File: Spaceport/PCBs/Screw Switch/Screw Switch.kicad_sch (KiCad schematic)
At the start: 2 parts

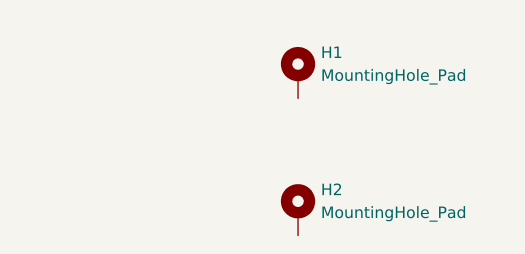
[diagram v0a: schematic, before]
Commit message: Update Screw Switch PCB and schematic files
- Increased pad dimensions in Screw Switch PCB from 3.8mm to 9.0mm for improved soldering and stability.
- Added a new mounting hole symbol in the Screw Switch schematic with properties for reference, value, footprint, datasheet, and description.
- Created an auto-saved file entry for the STM32 flight computer project to ensure recovery of recent changes.
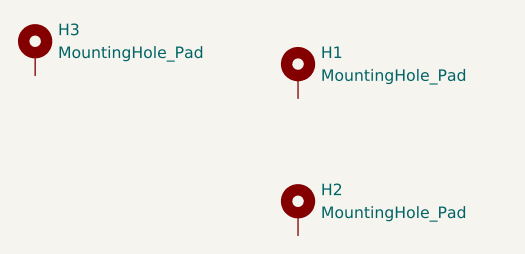
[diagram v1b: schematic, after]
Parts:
- added H3: MountingHole_Pad, MountingHole:MountingHole_3.2mm_M3_Pad_TopBottom, symbol Mechanical:MountingHole_Pad
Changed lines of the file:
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@@
+	(symbol
+		(lib_id "Mechanical:MountingHole_Pad")
+		(at 82.55 68.58 0)
+		(unit 1)
+		(exclude_from_sim yes)
+		(in_bom no)
+		(on_board yes)
+		(dnp no)
+		(fields_autoplaced yes)
+		(property "Reference" "H3"
+			(at 85.09 66.0399 0)
+			(effects
+				(font
+					(size 1.27 1.27)
+				)
+				(justify left)
+			)
+		)
+		(property "Value" "MountingHole_Pad"
+			(at 85.09 68.5799 0)
+			(effects
+				(font
+					(size 1.27 1.27)
+				)
+				(justify left)
+			)
+		)
+		(property "Footprint" "MountingHole:MountingHole_3.2mm_M3_Pad_TopBottom"
+			(at 82.55 68.58 0)
+			(effects
+				(font
+					(size 1.27 1.27)
+				)
+				(hide yes)
+			)
+		)
+		(property "Datasheet" "~"
+			(at 82.55 68.58 0)
+			(effects
+				(font
+					(size 1.27 1.27)
+				)
+				(hide yes)
+			)
+		)
+		(property "Description" "Mounting Hole with connection"
+			(at 82.55 68.58 0)
+			(effects
+				(font
+					(size 1.27 1.27)
+				)
+				(hide yes)
+			)
+		)
+		(pin "1"
+		)
+		(instances
+			(project "Screw Switch"
+				(path "/95d75f6d-4b6e-4fd0-917d-ccbce393357a"
+					(reference "H3")
+					(unit 1)
+				)
+			)
+		)
+	)
 	(symbol
 		(lib_id "Mechanical:MountingHole_Pad")
